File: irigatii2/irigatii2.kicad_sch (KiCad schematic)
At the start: 19 parts, among them J1 Screw_Terminal_01x02, J2 Conn_01x05

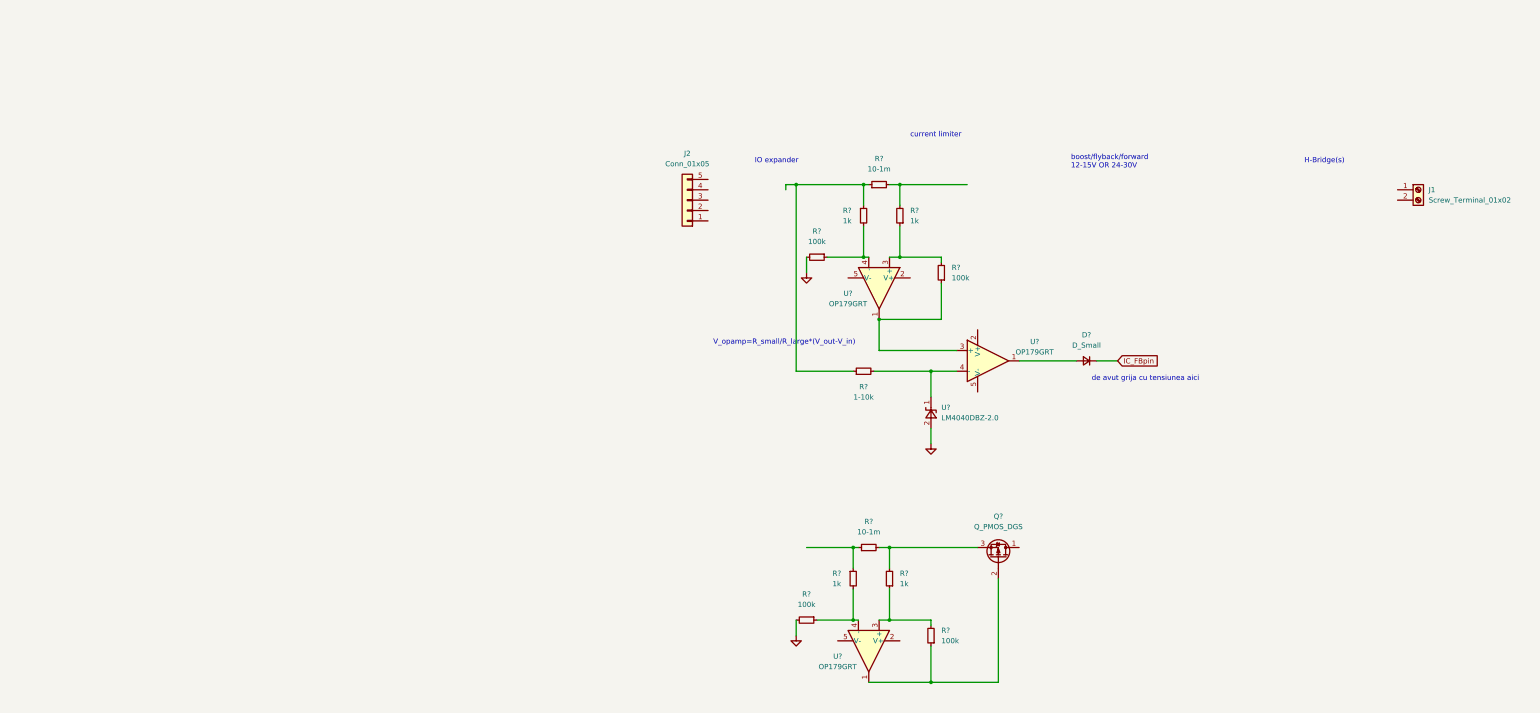
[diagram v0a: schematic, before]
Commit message: Update irigatii2.kicad_sch
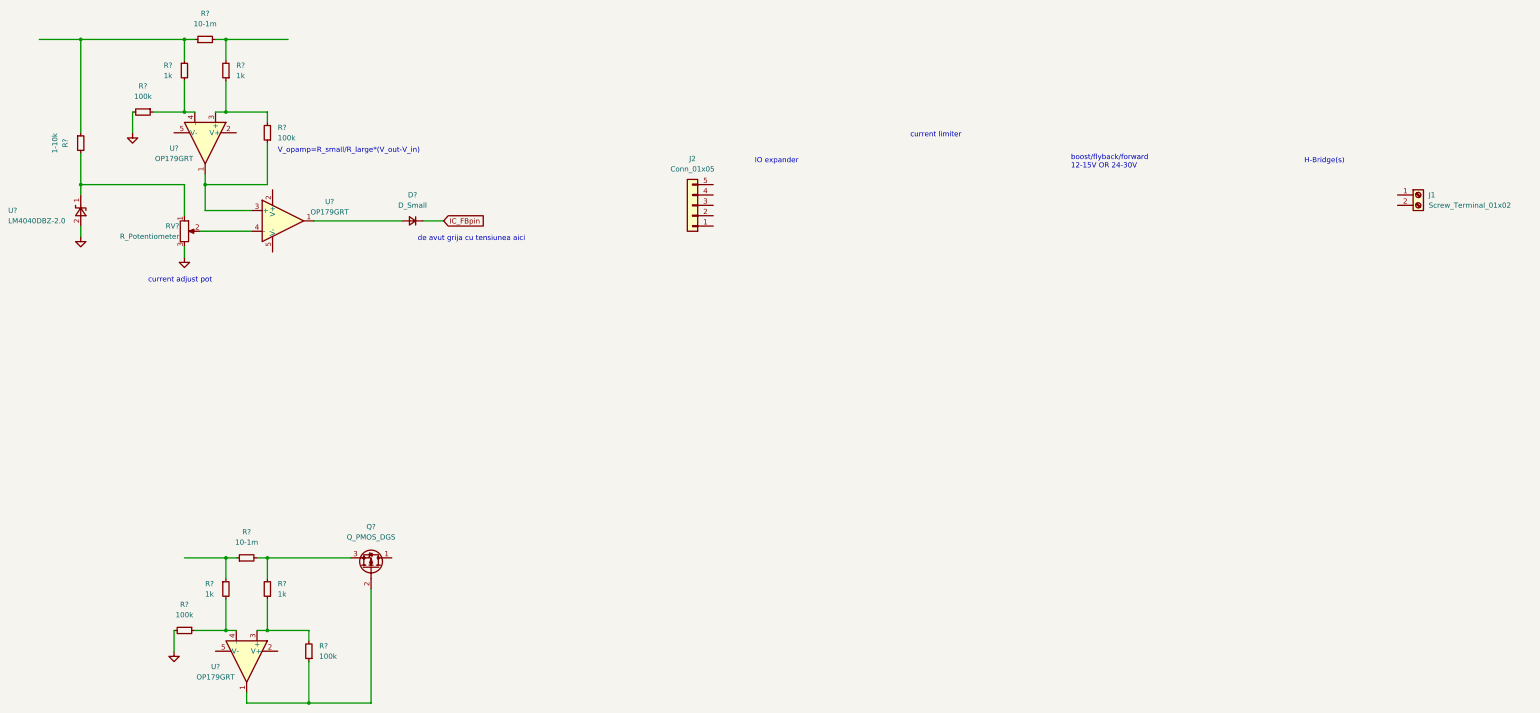
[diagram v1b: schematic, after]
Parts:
- added RV?: R_Potentiometer, symbol Device:R_Potentiometer
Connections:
- net GND: now also RV?.3
- net at R?.2, U?.1 (K): now also RV?.1; no longer U?.4 (-)
- new net: RV?.2, U?.4 (-)
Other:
- note added: "current adjust pot"
- moved on the sheet: D?, J1, J2, Q?, R?, U?

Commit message: t
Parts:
- removed Q?: Q_PMOS_DGS, symbol Device:Q_PMOS_DGS
- removed R? (x2): 100k, symbol Device:R_Small
- removed R? (x2): 1k, symbol Device:R_Small
- removed R?: 10-1m, symbol Device:R_Small
- removed U?: OP179GRT, Package_TO_SOT_SMD:SOT-23-5, symbol Amplifier_Operational:OP179GRT
- added C1, C2, C3, C4, C5, C6: C_Small, symbol Device:C_Small
- added C10, C9: 100n, symbol Device:C_Small
- added C7, C8: 1u, symbol Device:C_Small
- added D2, D3: D_Small, symbol Device:D_Small
- added IC1: MIC3172YN, DIP762W57P254L952H343Q8N, symbol SamacSys_Parts:MIC3172YN
- added IC2: PCA9575PW2,118, SOP65P640X110-28N, symbol SamacSys_Parts:PCA9575PW2,118
- added JP1, JP2, JP3, JP4: Adress0, Jumper:SolderJumper-3_P1.3mm_Bridged12_Pad1.0x1.5mm, symbol Jumper:Jumper_3_Bridged12
- added R1, R3, R4, R9: 100k, symbol Device:R_Small
- added R7: 1k, symbol Device:R_Small
- added T1: Transformer_1P_1S, symbol Device:Transformer_1P_1S
- R2: renamed from R?; value 10-1m -> 10m
- gave numbers to parts that had none: 10
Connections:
- net GND: now also J2.1 (Pin_1), C1.2, C10.2, C3.2, C4.2, C5.2, C6.1, C8.2, C9.2, IC1.1 (S_GND), IC1.6 (P_GND_2), IC1.8 (P_GND_1), IC2.16 (VSS), JP1.1 (A), JP2.1 (A), JP3.1 (A), JP4.1 (A), R4.1, R7.1, T1.3 (SA)
- net IC_FBpin: now also IC1.3 (FB), R3.1, R4.2
- net 2V: now reaches R11.2, RV1.1, U3.1 (K)
- net at R2.2, R6.2: now also C2.1, C6.2, IC1.5 (VIN), R1.2, T1.1 (AA)
- net I2C_CLK: now reaches J2.2 (Pin_2)
- net I2C_CLK: now also IC2.28 (SCL)
- net I2C_SDA: now reaches J2.3 (Pin_3)
- net I2C_SDA: now also IC2.27 (SDA)
- net +5V: now reaches J2.4 (Pin_4)
- net +3V3: now reaches J2.5 (Pin_5)
- net +3V3: now also C10.1, C8.1, C9.1, IC2.2 (VDD), IC2.21 (VDD(IO)1), IC2.9 (VDD(IO)0), JP1.3 (B), JP2.3 (B), JP3.3 (B), JP4.3 (B), R9.2
- new net: C1.1, C3.1, C4.1, C5.1, D2.1 (K), R3.2
- new net: D3.2 (A), IC1.7 (VSW), T1.2 (AB)
- new net: D2.2 (A), T1.4 (SB)
- new net: C2.2, D3.1 (K), R1.1
- new net: C7.1, IC1.2 (COMP)
- new net: C7.2, R7.2
- new net: IC2.3 (~{RESET}), R9.1
- new net A0: IC2.1 (A0), JP1.2 (C)
- new net A1: IC2.8 (A1), JP2.2 (C)
- new net A2: IC2.15 (A2), JP3.2 (C)
- new net A3: IC2.22 (A3), JP4.2 (C)
- no-connect marks 0 -> 1
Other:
- note added: "12V/24V"
- note added: "I2C adress: [0 1 0 A3 A2 A1 A0] gnd=0 vdd=1"
- note added: "IN: 2.5-3.3V OUT:12-24V max ratio 1/10 min ratio 1/3.6 (0.27) for 12V only: 1/4.8 (0.20)"
- note added: "V_opamp=R_small/R_large*(V_out-V_in) r=10m => 300mA->300mV"
- note removed: "V_opamp=R_small/R_large*(V_out-V_in)"
- note removed: "boost/flyback/forward 12-15V OR 24-30V"
- note removed: "de avut grija cu tensiunea aici"
- moved on the sheet: D1, R10, R11, R2, R5, R6, R8, RV1, U2, U3, U4

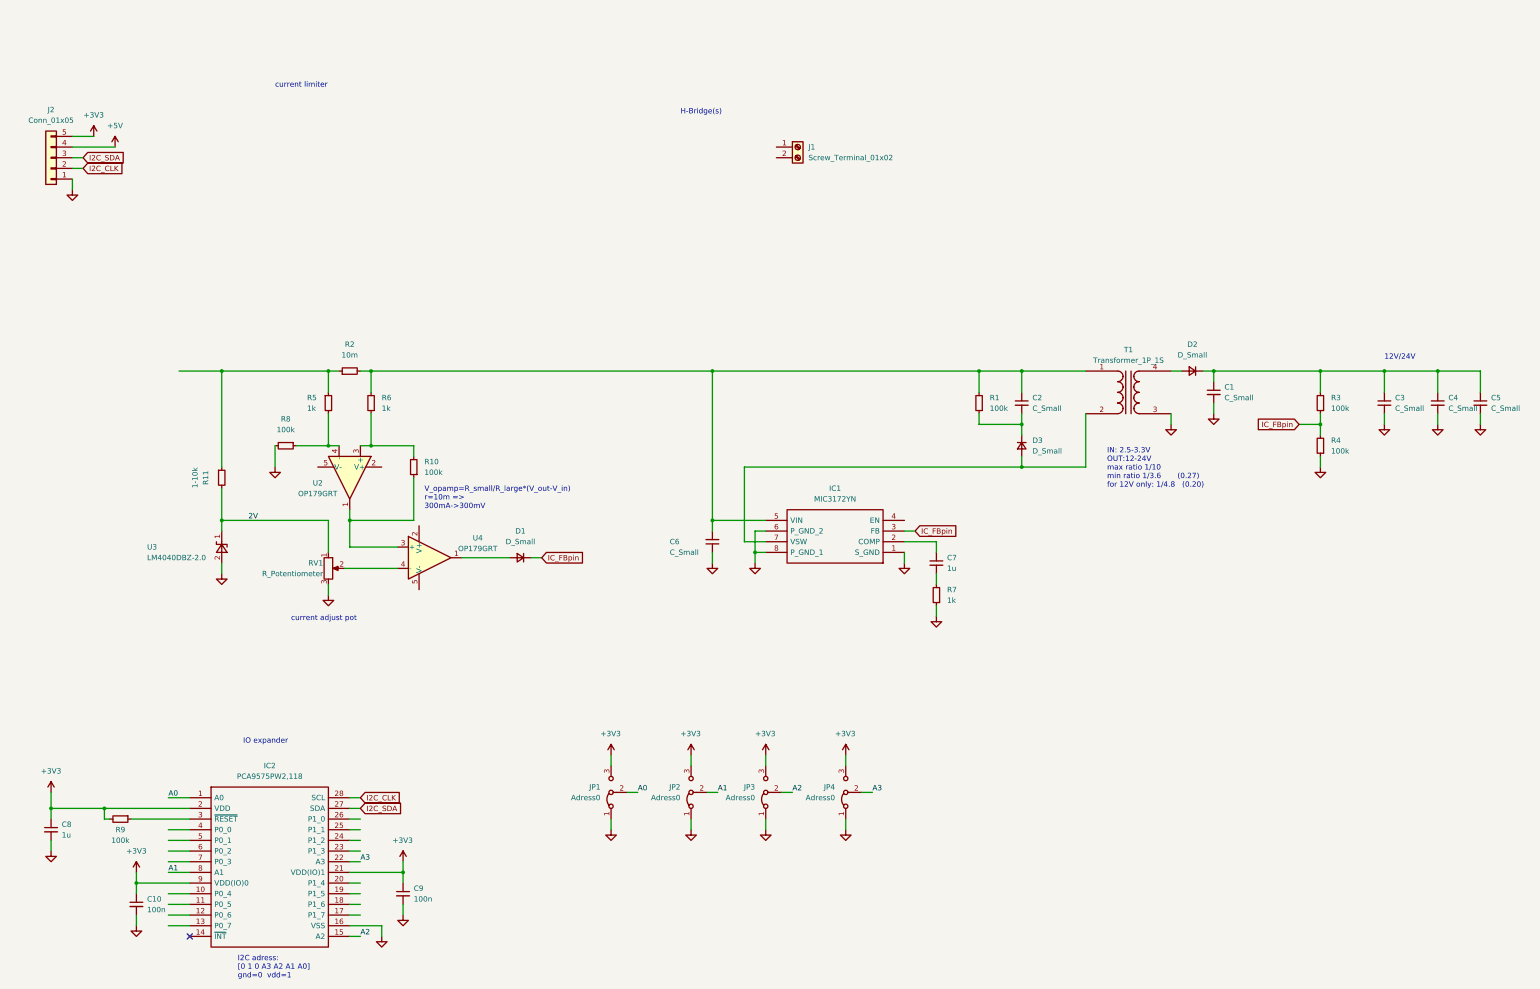
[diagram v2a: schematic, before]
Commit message: g
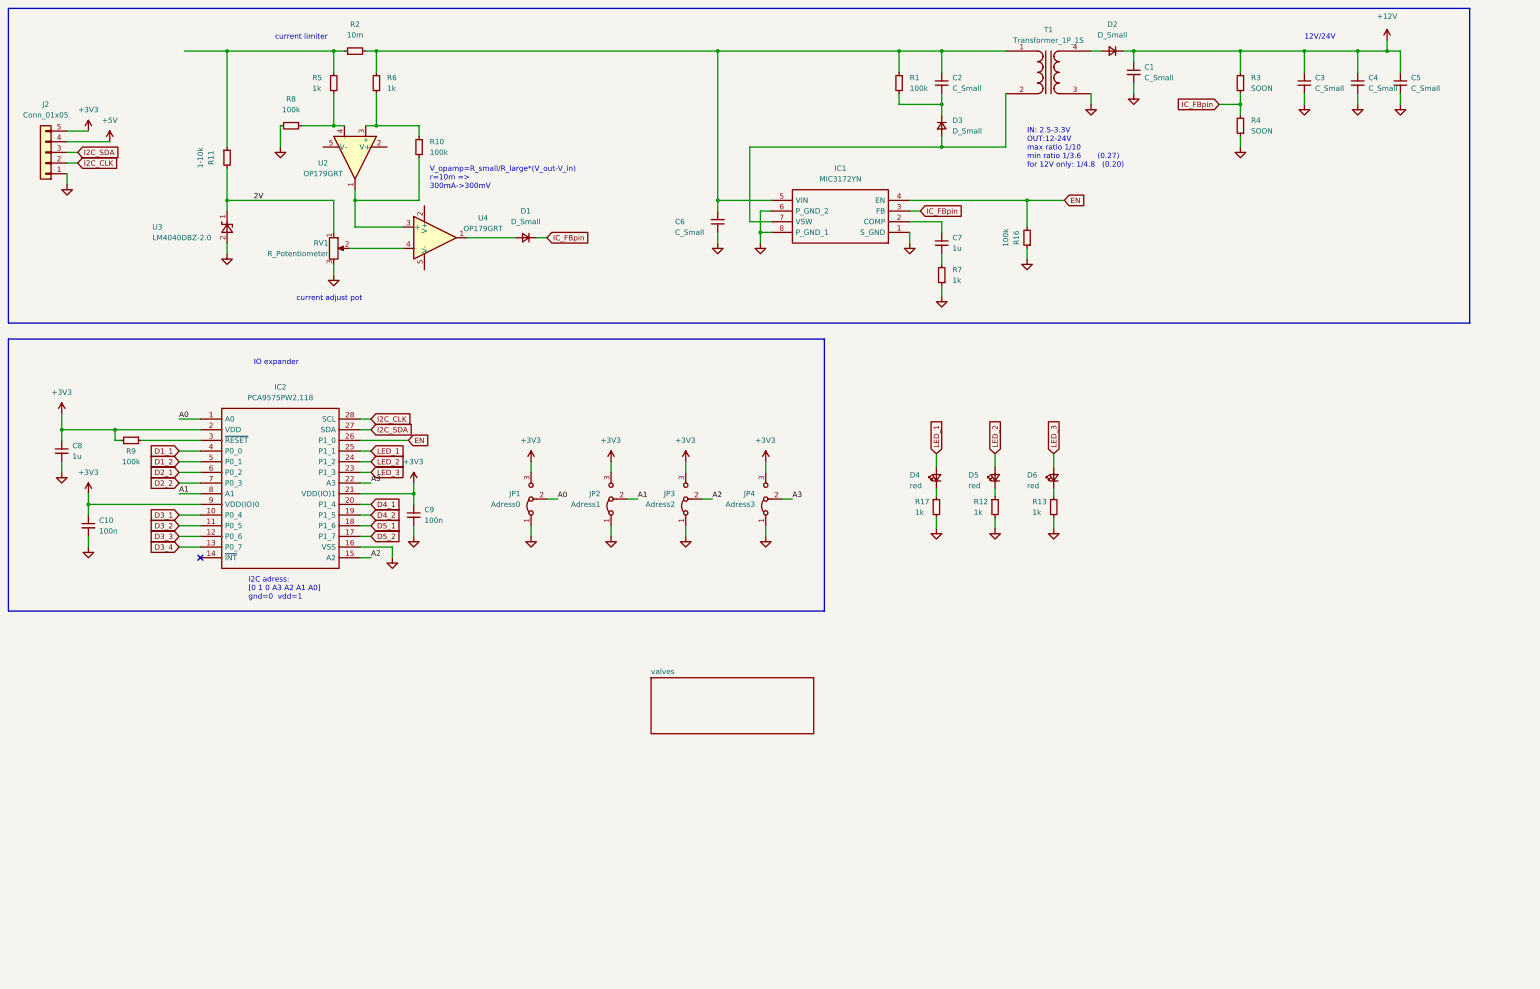
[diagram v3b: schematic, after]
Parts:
- removed J1: Screw_Terminal_01x02, TerminalBlock:TerminalBlock_Altech_AK300-2_P5.00mm, symbol Connector:Screw_Terminal_01x02
- added D4, D5, D6: red, LED_THT:LED_D5.0mm, symbol Device:LED_Small
- added R12, R13, R17: 1k, Resistor_THT:R_Axial_DIN0207_L6.3mm_D2.5mm_P10.16mm_Horizontal, symbol Device:R_Small
- added R16: 100k, Resistor_THT:R_Axial_DIN0207_L6.3mm_D2.5mm_P10.16mm_Horizontal, symbol Device:R_Small
- C1, C2, C3, C4, C5, C6: footprint (none) -> Capacitor_THT:CP_Axial_L11.0mm_D5.0mm_P18.00mm_Horizontal
- C10, C7, C8, C9: footprint (none) -> Capacitor_THT:C_Disc_D3.8mm_W2.6mm_P2.50mm
- D1, D2, D3: footprint (none) -> Diode_THT:D_A-405_P5.08mm_Vertical_KathodeUp
- IC1: footprint DIP762W57P254L952H343Q8N -> SamacSys_Parts:DIP762W57P254L952H343Q8N
- IC2: footprint SOP65P640X110-28N -> SamacSys_Parts:SOP65P640X110-28N
- JP2: value Adress0 -> Adress1
- JP3: value Adress0 -> Adress2
- JP4: value Adress0 -> Adress3
- R1, R10, R11, R2, R5, R6, R7, R8, R9: footprint (none) -> Resistor_THT:R_Axial_DIN0207_L6.3mm_D2.5mm_P10.16mm_Horizontal
- R3, R4: value 100k -> SOON; footprint (none) -> Resistor_THT:R_Axial_DIN0207_L6.3mm_D2.5mm_P10.16mm_Horizontal
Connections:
- net GND: now also R12.2, R13.2, R16.1, R17.2
- net +12V: now reaches C1.1, C3.1, C4.1, C5.1, D2.1 (K), R3.2
- net EN: now reaches IC1.4 (EN)
- net EN: now also IC2.26 (P1_0), R16.2
- net D3_1: now reaches IC2.10 (P0_4)
- net D3_2: now reaches IC2.11 (P0_5)
- net D3_3: now reaches IC2.12 (P0_6)
- net D3_4: now reaches IC2.13 (P0_7)
- net D5_2: now reaches IC2.17 (P1_7)
- net D5_1: now reaches IC2.18 (P1_6)
- net D4_2: now reaches IC2.19 (P1_5)
- net D4_1: now reaches IC2.20 (P1_4)
- net LED_3: now reaches IC2.23 (P1_3)
- net LED_3: now also D6.2 (A)
- net LED_2: now reaches IC2.24 (P1_2)
- net LED_2: now also D5.2 (A)
- net LED_1: now reaches IC2.25 (P1_1)
- net LED_1: now also D4.2 (A)
- net D1_1: now reaches IC2.4 (P0_0)
- net D1_2: now reaches IC2.5 (P0_1)
- net D2_1: now reaches IC2.6 (P0_2)
- net D2_2: now reaches IC2.7 (P0_3)
- new net: D5.1 (K), R12.1
- new net: D4.1 (K), R17.1
- new net: D6.1 (K), R13.1
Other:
- added sheet valves (untitled.kicad_sch)
- note removed: "H-Bridge(s)"
- moved on the sheet: C1, C10, C2, C3, C4, C5, C6, C7, C8, C9, D1, D2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

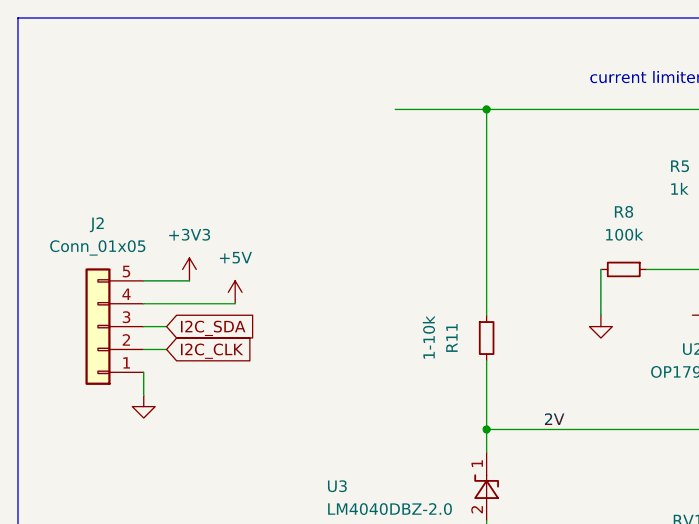
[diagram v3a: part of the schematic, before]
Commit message: h
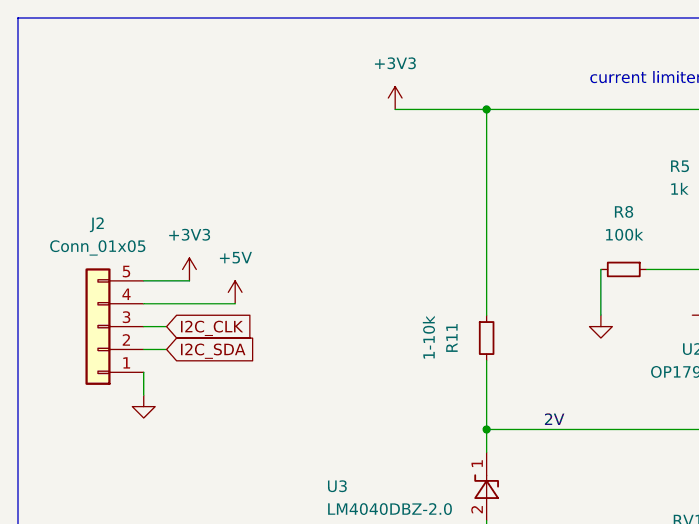
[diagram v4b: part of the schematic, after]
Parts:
- RV1: footprint (none) -> Potentiometer_THT:Potentiometer_ACP_CA9-V10_Vertical
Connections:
- net +3V3: now also R11.1, R2.1, R5.1
- net I2C_CLK: now also J2.3 (Pin_3); no longer J2.2 (Pin_2)
- net I2C_SDA: now also J2.2 (Pin_2); no longer J2.3 (Pin_3)
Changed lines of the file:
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@@
     )
   )
-  (global_label "I2C_SDA" (shape input) (at 31.75 49.53 0) (fields_autoplaced)
+  (global_label "I2C_SDA" (shape input) (at 31.75 52.07 0) (fields_autoplaced)
     (effects (font (size 1.27 1.27)) (justify left))
-    (property "Intersheet References" "${INTERSHEET_REFS}" (id 0) (at 41.7831 49.4506 0)
+    (property "Intersheet References" "${INTERSHEET_REFS}" (id 0) (at 41.7831 52.1494 0)
       (effects (font (size 1.27 1.27)) (justify left) hide)
     )
@@
     )
   )
-  (global_label "I2C_CLK" (shape input) (at 31.75 52.07 0) (fields_autoplaced)
+  (global_label "I2C_CLK" (shape input) (at 31.75 49.53 0) (fields_autoplaced)
     (effects (font (size 1.27 1.27)) (justify left))
-    (property "Intersheet References" "${INTERSHEET_REFS}" (id 0) (at 41.7831 51.9906 0)
+    (property "Intersheet References" "${INTERSHEET_REFS}" (id 0) (at 41.7831 49.6094 0)
       (effects (font (size 1.27 1.27)) (justify left) hide)
     )
@@
     )
     (property "Datasheet" "" (id 3) (at 176.53 140.97 0)
+      (effects (font (size 1.27 1.27)) hide)
+    )
+    (pin "1")
+  )
+  (symbol (lib_id "power:+3V3") (at 57.15 25.4 0) (unit 1)
+    (in_bom yes) (on_board yes) (fields_autoplaced)
+    (property "Reference" "#PWR0132" (id 0) (at 57.15 29.21 0)
+      (effects (font (size 1.27 1.27)) hide)
+    )
+    (property "Value" "+3V3" (id 1) (at 57.15 20.32 0))
+    (property "Footprint" "" (id 2) (at 57.15 25.4 0)
+      (effects (font (size 1.27 1.27)) hide)
+    )
+    (property "Datasheet" "" (id 3) (at 57.15 25.4 0)
       (effects (font (size 1.27 1.27)) hide)
     )
@@
       (effects (font (size 1.27 1.27)) (justify right))
     )
-    (property "Footprint" "" (id 2) (at 92.71 72.39 0)
+    (property "Footprint" "Potentiometer_THT:Potentiometer_ACP_CA9-V10_Vertical" (id 2) (at 92.71 72.39 0)
       (effects (font (size 1.27 1.27)) hide)
     )
@@
       (reference "#PWR0131") (unit 1) (value "GND") (footprint "")
     )
+    (path "/a946c6f8-1cd0-4f73-865c-8398351b54de"
+      (reference "#PWR0132") (unit 1) (value "+3V3") (footprint "")
+    )
     (path "/15ac21d5-9c0d-4dcf-b906-d2a3e2e6e333"
       (reference "#PWR0142") (unit 1) (value "+12V") (footprint "")
@@
     )
     (path "/f1636799-ee9a-41a3-9250-62c97be0fdd1"
-      (reference "RV1") (unit 1) (value "R_Potentiometer") (footprint "")
+      (reference "RV1") (unit 1) (value "R_Potentiometer") (footprint "Potentiometer_THT:Potentiometer_ACP_CA9-V10_Vertical")
     )
     (path "/204b8d26-cc7c-479f-ad89-06a91f5ab1e6"
